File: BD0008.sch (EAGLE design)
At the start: 9 parts, among them J1 HEADER_1X3MALE, J2 HEADER_1X3FEMALE

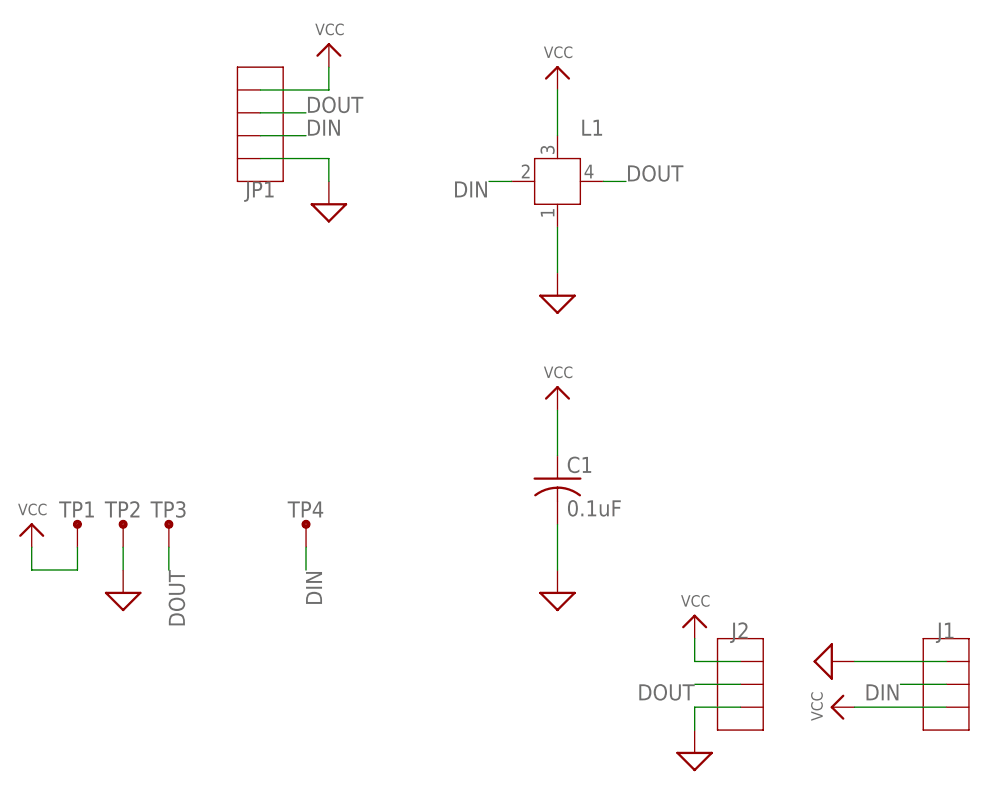
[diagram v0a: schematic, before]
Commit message: initial updates from v1. (not sure what was changed)
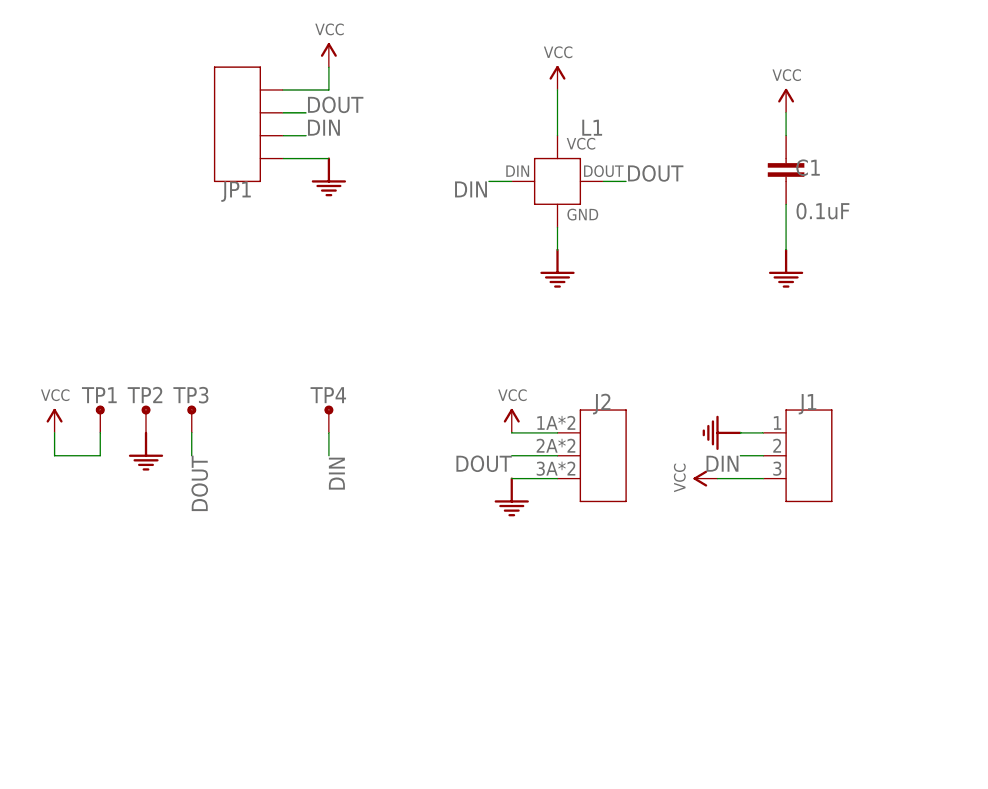
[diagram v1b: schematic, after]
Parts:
- C1: device adafruit:C-USC0402 -> DroidForge:CAPACITOR-0402
- J1: device Clock:HEADER_1X3MALE -> DroidForge:HEADER_1X3MALE
- J2: device Clock:HEADER_1X3FEMALE -> DroidForge:HEADER_1X3FEMALE
- JP1: value HEADER_1X4S -> HEADER_1X4; device Clock:HEADER_1X4S -> DroidForge:HEADER_1X4
- L1: value WS2812B -> WS2812B-B; device Clock:WS2812B -> DroidForge:WS2812B-B
- TP1, TP2, TP3, TP4: device Clock:TEST_POINT -> DroidForge:TEST_POINT
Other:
- moved on the sheet: C1, L1, TP1, TP2, TP3, TP4
